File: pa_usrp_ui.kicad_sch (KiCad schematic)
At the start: 18 parts, among them J1 BWSMA-KE-P001, J2 BWSMA-KE-P001, J3 2118722-2, U1 QPA9418TR13

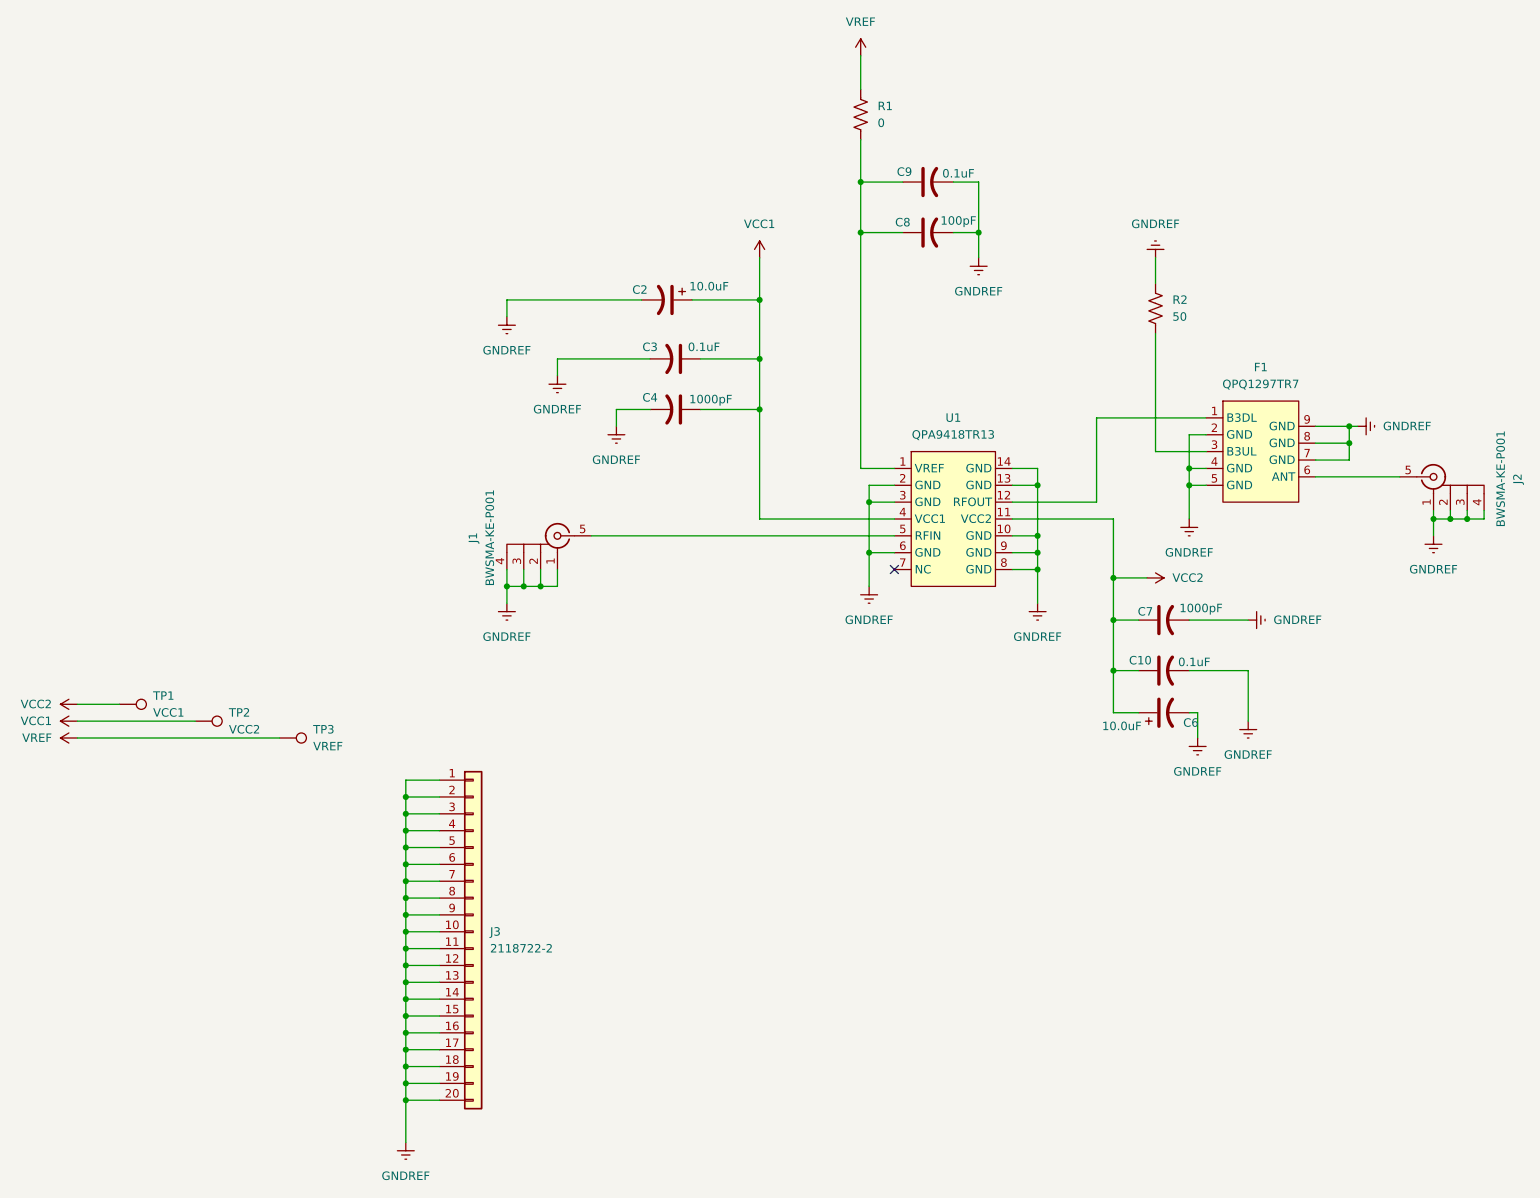
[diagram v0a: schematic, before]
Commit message: Adding lna uplink
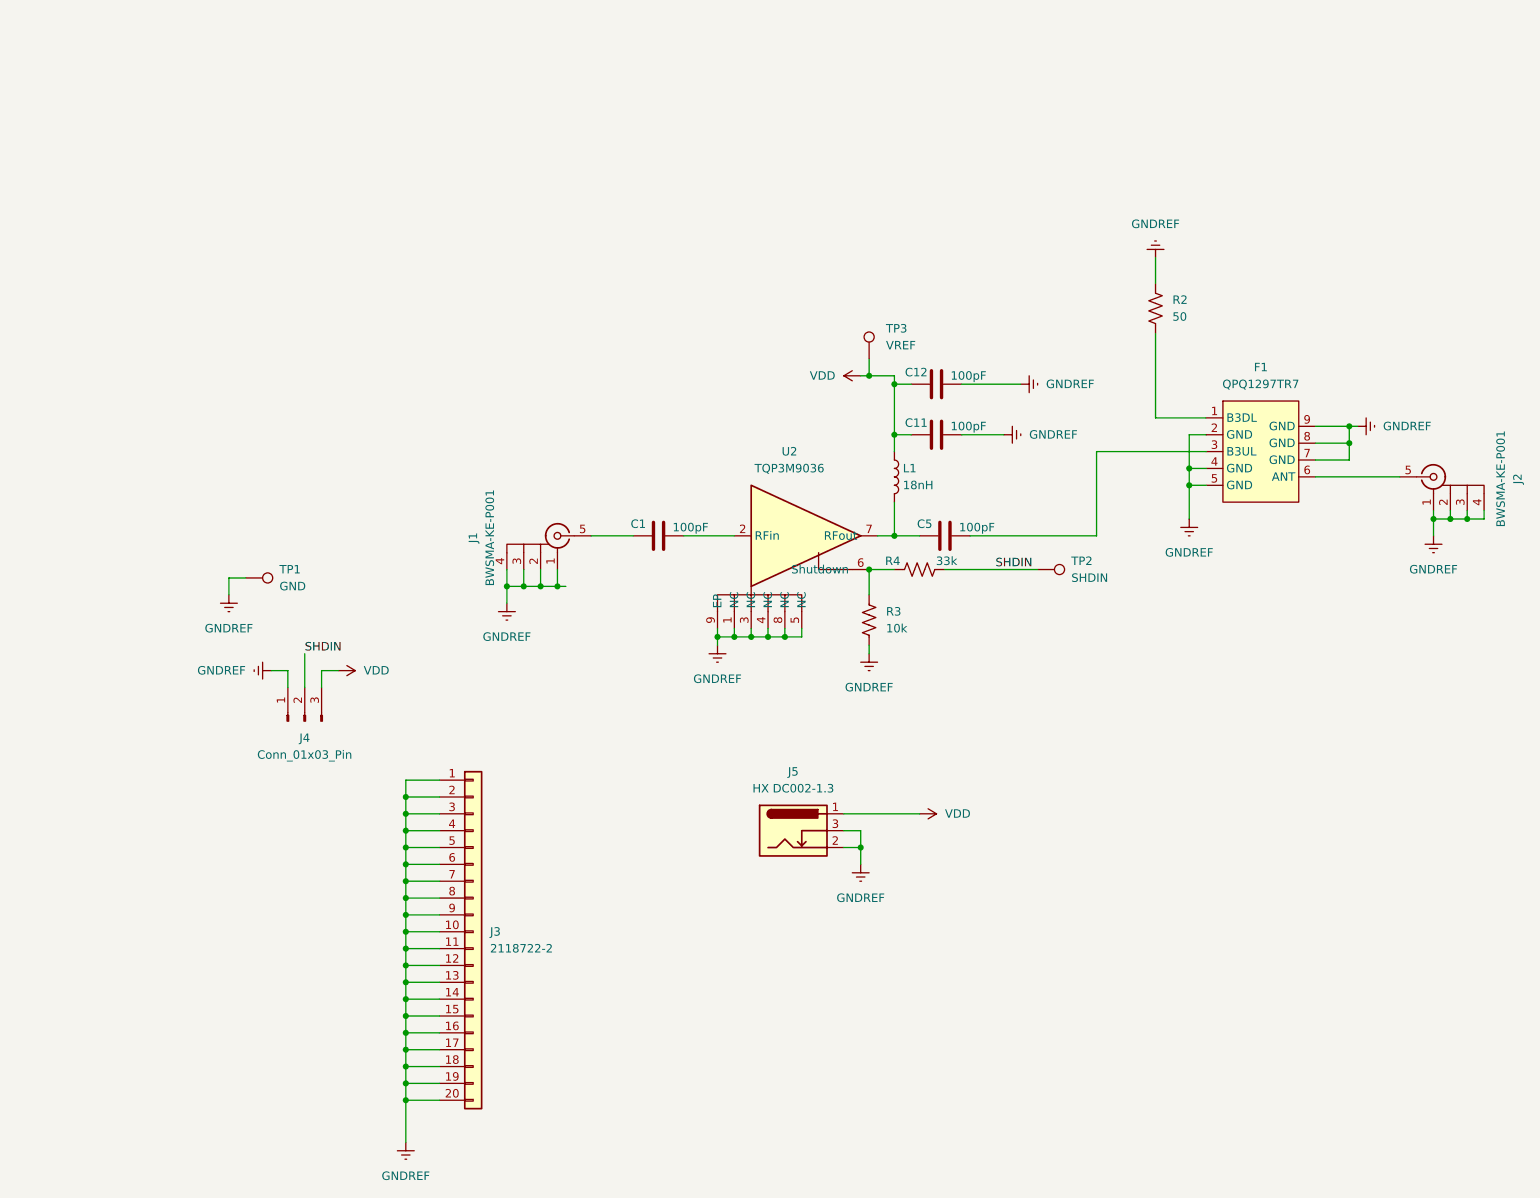
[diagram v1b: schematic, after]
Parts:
- removed C10, C3, C9: 0.1uF, Capacitor_SMD:C_0603_1608Metric, symbol Device:C_US
- removed C2, C6: 10.0uF, Diode_SMD:D_0603_1608Metric, symbol Device:C_Polarized_US
- removed C4, C7: 1000pF, Capacitor_SMD:C_0603_1608Metric, symbol Device:C_US
- removed C8: 100pF, Capacitor_SMD:C_0603_1608Metric, symbol Device:C_US
- removed R1: 0, Resistor_SMD:R_0603_1608Metric, symbol Device:R_US
- removed U1: QPA9418TR13, fooptrints:DFN-14_L7.0-W7.0-P1.06-TL-EP_QPA9418TR13, symbol pa_ui:QPA9418TR13
- added C1, C11, C12, C5: 100pF, Capacitor_SMD:C_0603_1608Metric, symbol Device:C
- added J4: Conn_01x03_Pin, Connector_PinHeader_2.54mm:PinHeader_1x03_P2.54mm_Vertical, symbol Connector:Conn_01x03_Pin
- added J5: HX DC002-1.3, fooptrints:DC-IN-TH_HANXIA_HX-DC002-1.3, symbol Connector:Barrel_Jack_Switch
- added L1: 18nH, Inductor_SMD:L_0603_1608Metric, symbol Device:L
- added R3: 10k, Resistor_SMD:R_0603_1608Metric, symbol Device:R_US
- added R4: 33k, Resistor_SMD:R_0603_1608Metric, symbol Device:R_US
- added U2: TQP3M9036, fooptrints:DFN-8_L2.0-W2.0-P0.50-BL-EP, symbol pa_ui:TQP3M9036
- TP1: value VCC1 -> GND
- TP2: value VCC2 -> SHDIN
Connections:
- net VCC2 is gone; now on net GNDREF: TP1.1
- net GNDREF: now also C11.2, C12.2, J4.1 (Pin_1), J5.2, J5.3, R3.2, U2.1 (NC), U2.3 (NC), U2.4 (NC), U2.5 (NC), U2.8 (NC), U2.9 (EP)
- net at F1.1 (B3DL): now also R2.2
- net at F1.3 (B3UL): now also C5.2; no longer R2.2
- net at J1.5: now also C1.1
- net VCC1 renamed SHDIN
- net SHDIN: now also J4.2 (Pin_2), R4.2
- net VREF renamed VDD
- net VDD: now also C11.1, C12.1, J4.3 (Pin_3), J5.1, L1.1
- new net: R3.1, R4.1, U2.6 (Shutdown)
- new net: C5.1, L1.2, U2.7 (RFout)
- new net: C1.2, U2.2 (RFin)
- no-connect marks 1 -> 0
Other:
- moved on the sheet: TP3
